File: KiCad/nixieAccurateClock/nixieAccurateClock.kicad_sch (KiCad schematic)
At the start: 7 parts, among them J1 Conn_01x02_Pin, J2 Conn_01x02_Pin, J3 Conn_01x02_Pin, SW1 SW_DIP_x02

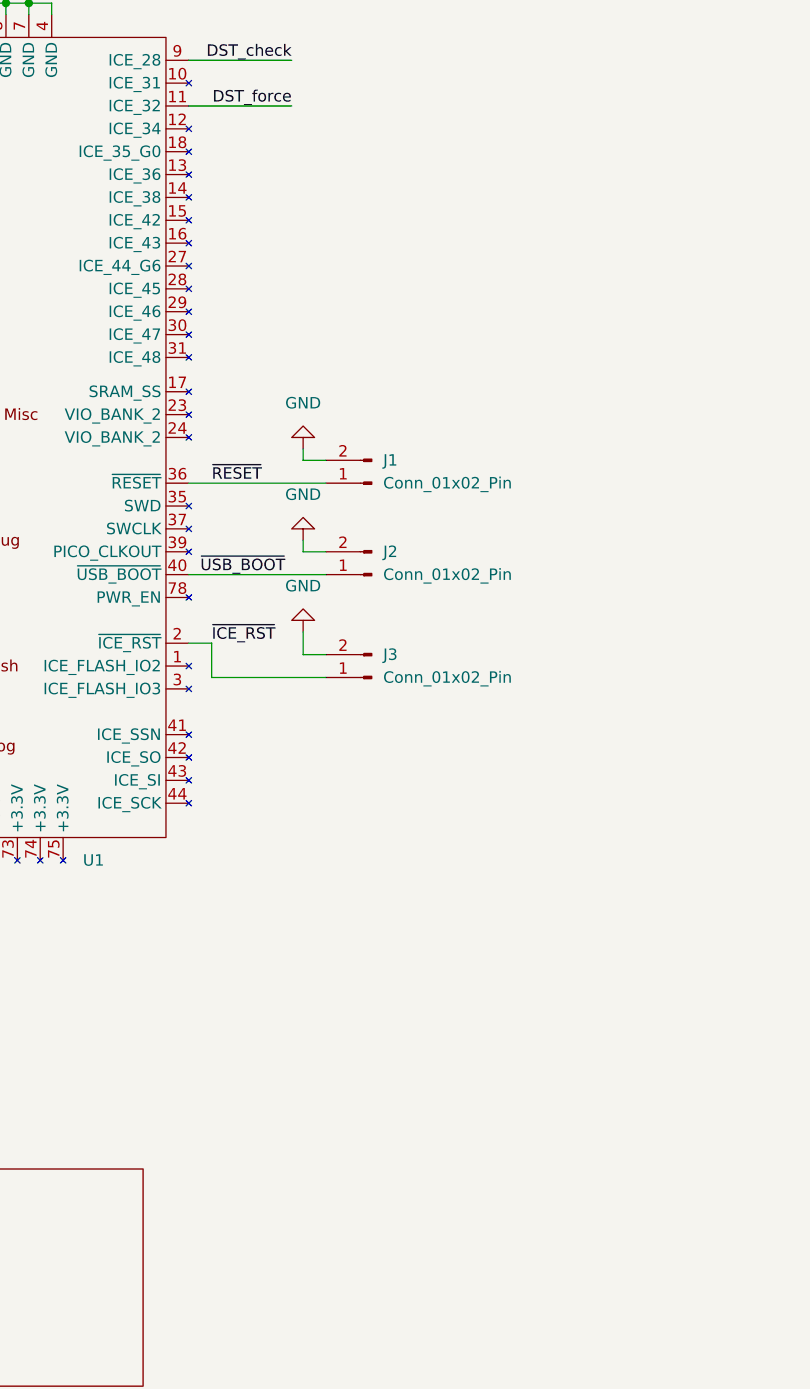
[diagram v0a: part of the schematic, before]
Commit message: WIP nixies
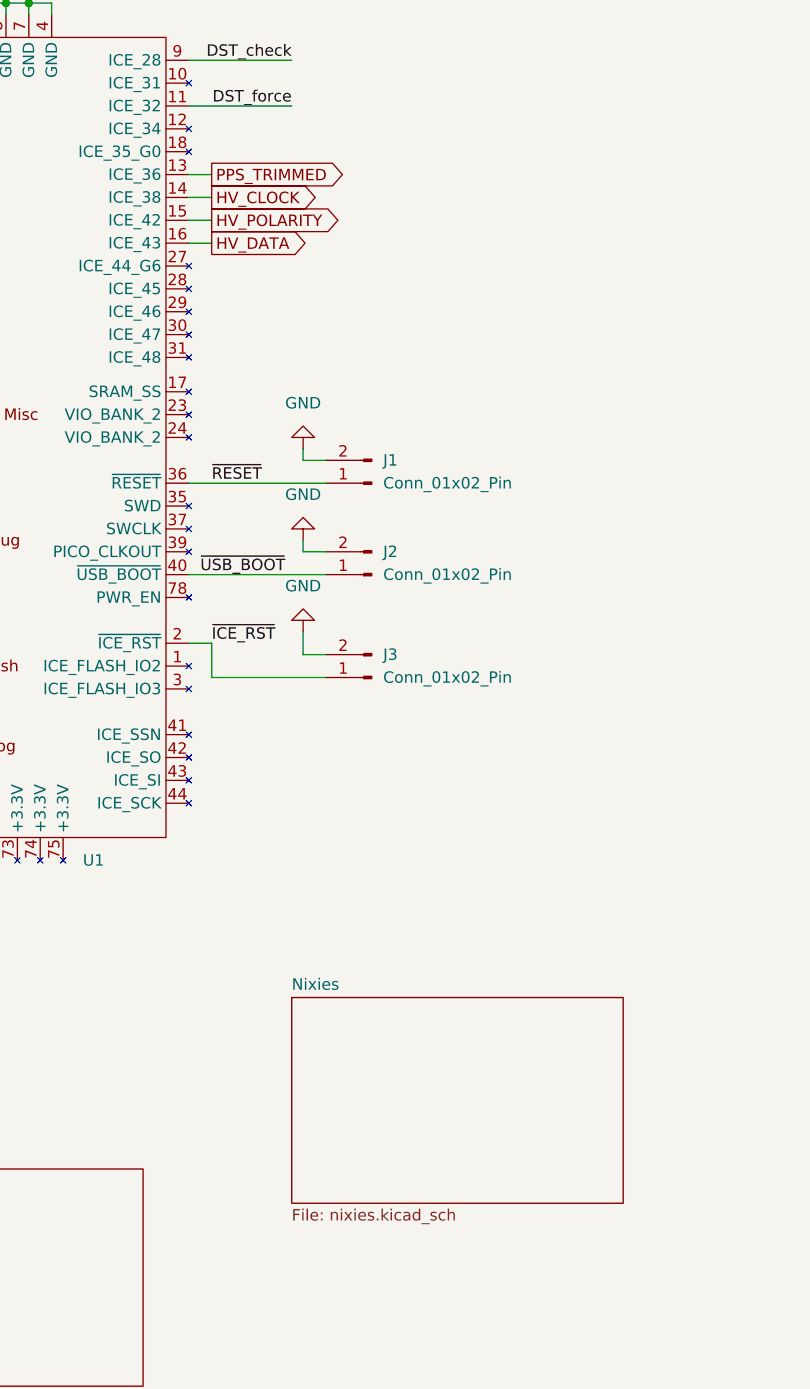
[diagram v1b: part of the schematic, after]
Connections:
- net PPS_TRIMMED: now reaches U1.13 (ICE_36)
- net HV_CLOCK: now reaches U1.14 (ICE_38)
- net HV_POLARITY: now reaches U1.15 (ICE_42)
- net HV_DATA: now reaches U1.16 (ICE_43)
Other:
- added sheet Nixies (nixies.kicad_sch)
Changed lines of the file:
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@@
+    (stroke (width 0) (type default))
+  )
+  (wire (pts (xy 134.62 48.26) (xy 137.16 48.26))
+    (stroke (width 0) (type default))
+  )
+  (wire (pts (xy 134.62 40.64) (xy 137.16 40.64))
     (stroke (width 0) (type default))
   )
@@
     (stroke (width 0) (type default))
   )
+  (wire (pts (xy 134.62 43.18) (xy 137.16 43.18))
+    (stroke (width 0) (type default))
+  )
   (wire (pts (xy 149.86 72.39) (xy 147.32 72.39))
     (stroke (width 0) (type default))
@@
   )
   (wire (pts (xy 134.62 33.02) (xy 146.05 33.02))
+    (stroke (width 0) (type default))
+  )
+  (wire (pts (xy 134.62 45.72) (xy 137.16 45.72))
     (stroke (width 0) (type default))
   )
@@
     )
   )
+  (global_label "HV_CLOCK" (shape output) (at 137.16 43.18 0) (fields_autoplaced)
+    (effects (font (size 1.27 1.27)) (justify left))
+    (property "Intersheetrefs" "${INTERSHEET_REFS}" (at 149.7005 43.18 0)
+      (effects (font (size 1.27 1.27)) (justify left) hide)
+    )
+  )
+  (global_label "HV_POLARITY" (shape output) (at 137.16 45.72 0) (fields_autoplaced)
+    (effects (font (size 1.27 1.27)) (justify left))
+    (property "Intersheetrefs" "${INTERSHEET_REFS}" (at 152.1801 45.72 0)
+      (effects (font (size 1.27 1.27)) (justify left) hide)
+    )
+  )
   (global_label "GPS_BOOT_SEL" (shape output) (at 72.39 68.58 180) (fields_autoplaced)
     (effects (font (size 1.27 1.27)) (justify right))
@@
     )
   )
+  (global_label "PPS_TRIMMED" (shape output) (at 137.16 40.64 0) (fields_autoplaced)
+    (effects (font (size 1.27 1.27)) (justify left))
+    (property "Intersheetrefs" "${INTERSHEET_REFS}" (at 153.0265 40.64 0)
+      (effects (font (size 1.27 1.27)) (justify left) hide)
+    )
+  )
   (global_label "GPS_1PPS" (shape input) (at 71.12 50.8 180) (fields_autoplaced)
     (effects (font (size 1.27 1.27)) (justify right))
@@
     (property "Intersheetrefs" "${INTERSHEET_REFS}" (at 57.2492 45.72 0)
       (effects (font (size 1.27 1.27)) (justify right) hide)
+    )
+  )
+  (global_label "HV_DATA" (shape output) (at 137.16 48.26 0) (fields_autoplaced)
+    (effects (font (size 1.27 1.27)) (justify left))
+    (property "Intersheetrefs" "${INTERSHEET_REFS}" (at 147.9467 48.26 0)
+      (effects (font (size 1.27 1.27)) (justify left) hide)
     )
   )
@@
       )
     )
+  )
+  (sheet (at 146.05 132.08) (size 36.83 22.86) (fields_autoplaced)
+    (stroke (width 0.1524) (type solid))
+    (fill (color 0 0 0 0.0000))
+    (property "Sheetname" "Nixies" (at 146.05 131.3684 0)
+      (effects (font (size 1.27 1.27)) (justify left bottom))
+    )
+    (property "Sheetfile" "nixies.kicad_sch" (at 146.05 155.5246 0)
+      (effects (font (size 1.27 1.27)) (justify left top))
+    )
+    (instances
+      (project "nixieAccurateClock"
+        (path "/55aab698-7558-4fe2-95ad-faa6da60ef89" (page "4"))
+      )
+    )
